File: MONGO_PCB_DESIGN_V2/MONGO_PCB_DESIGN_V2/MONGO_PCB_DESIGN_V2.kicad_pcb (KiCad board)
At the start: 2 copper layers, 100 x 98 mm, 6 parts

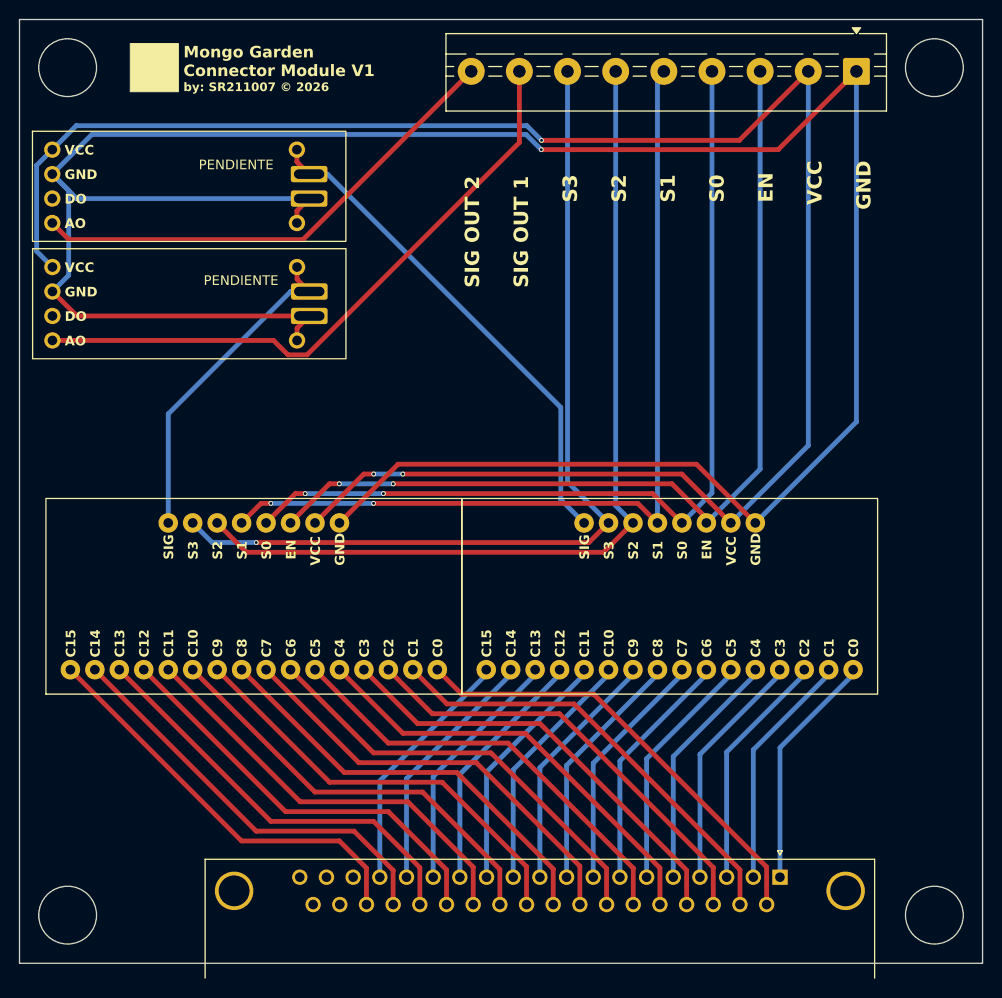
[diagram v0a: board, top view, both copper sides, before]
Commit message: PCB
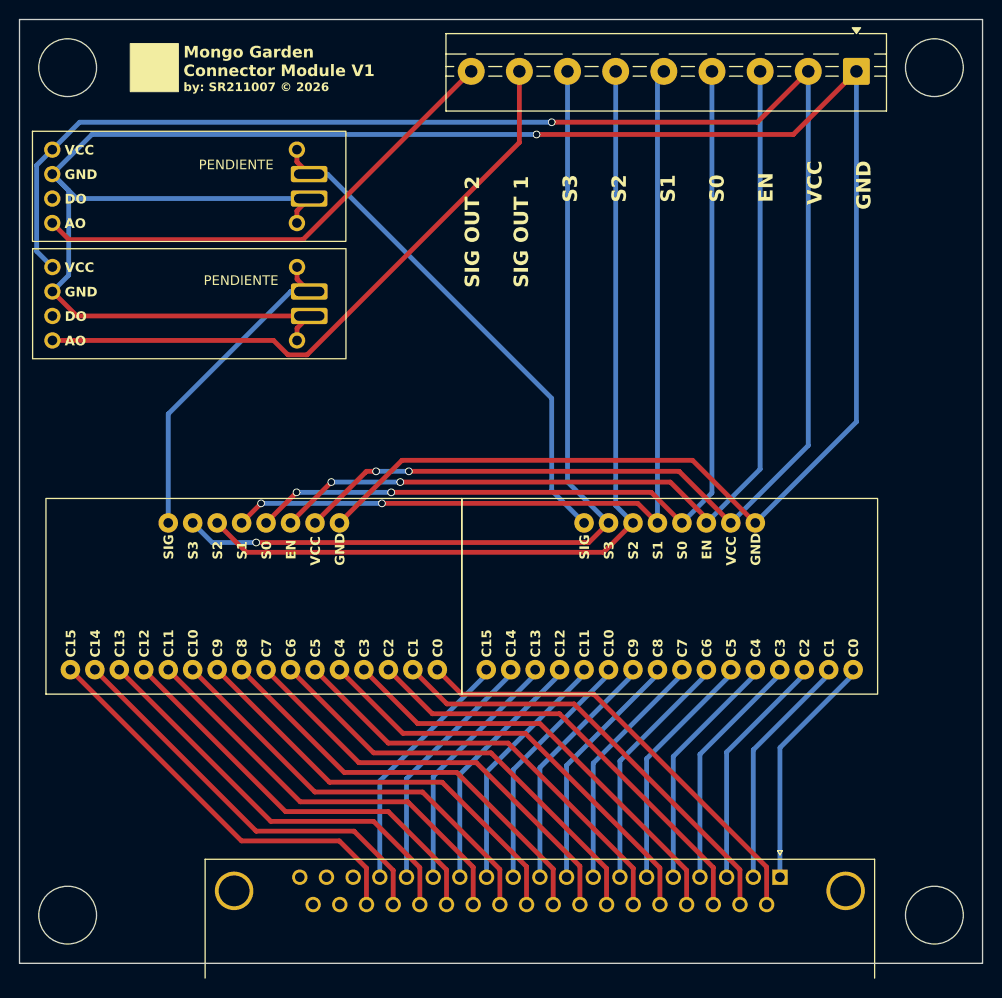
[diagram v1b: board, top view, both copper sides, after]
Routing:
- net VCC: track 194.3 -> 193.3 mm
- net GND: track 263.9 -> 262.9 mm
